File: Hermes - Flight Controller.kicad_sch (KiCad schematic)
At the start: 1 part

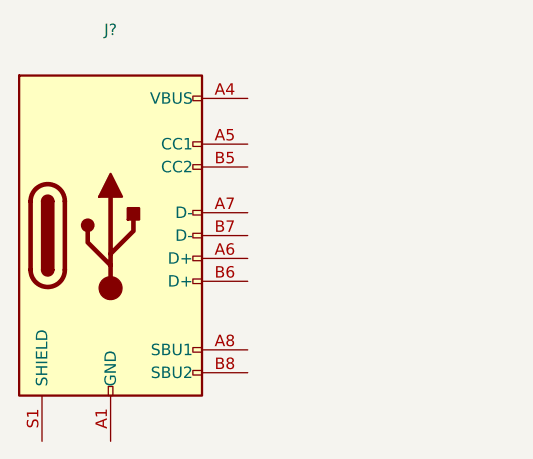
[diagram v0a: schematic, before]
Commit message: connector
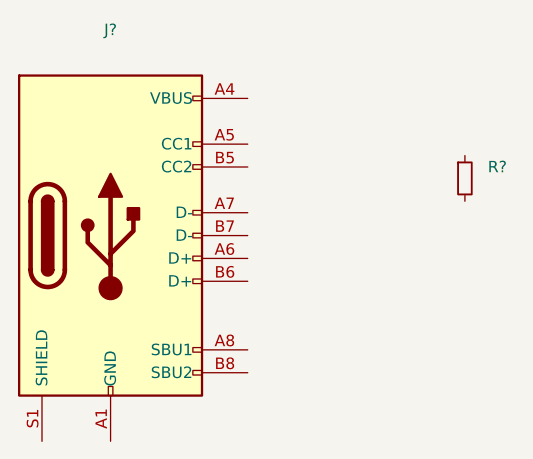
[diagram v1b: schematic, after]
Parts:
- added R?: (no value), symbol Device:R_Small
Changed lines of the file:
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@@
 (kicad_sch (version 20211123) (generator eeschema)
   (paper "A4")
+  (symbol (lib_id "Device:R_Small") (at 128.27 48.26 0) (unit 1)
+    (in_bom yes) (on_board yes) (fields_autoplaced)
+    (property "Reference" "R?" (id 0) (at 130.81 46.9899 0)
+      (effects (font (size 1.27 1.27)) (justify left))
+    )
+    (property "Value" "" (id 1) (at 130.81 49.5299 0)
+      (effects (font (size 1.27 1.27)) (justify left))
+    )
+    (property "Footprint" "" (id 2) (at 128.27 48.26 0)
+      (effects (font (size 1.27 1.27)) hide)
+    )
+    (property "Datasheet" "~" (id 3) (at 128.27 48.26 0)
+      (effects (font (size 1.27 1.27)) hide)
+    )
+    (pin "1")
+    (pin "2")
+  )
   (symbol (lib_id "Connector:USB_C_Receptacle_USB2.0") (at 88.9 54.61 0) (unit 1)
     (in_bom yes) (on_board yes) (fields_autoplaced)
@@
       (reference "J?") (unit 1) (value "USB_C_Receptacle_USB2.0") (footprint "")
     )
+    (path "/d8f1aa4a-2f21-4570-b6e4-a5df899c3581"
+      (reference "R?") (unit 1) (value "R_Small") (footprint "")
+    )
   )
